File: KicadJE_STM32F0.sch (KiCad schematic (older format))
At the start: 101 parts, among them J401 CV1, J402 CV2, J403 OUT1, J404 OUT2, J405 OUT3, J406 OUT4, J407 IN1, J408 IN2, J409 I2C, P401 Doepfer_Power_16pin, SW401 SW_SPDT, U401 TL072, U402 TL072, U405 MCP4822

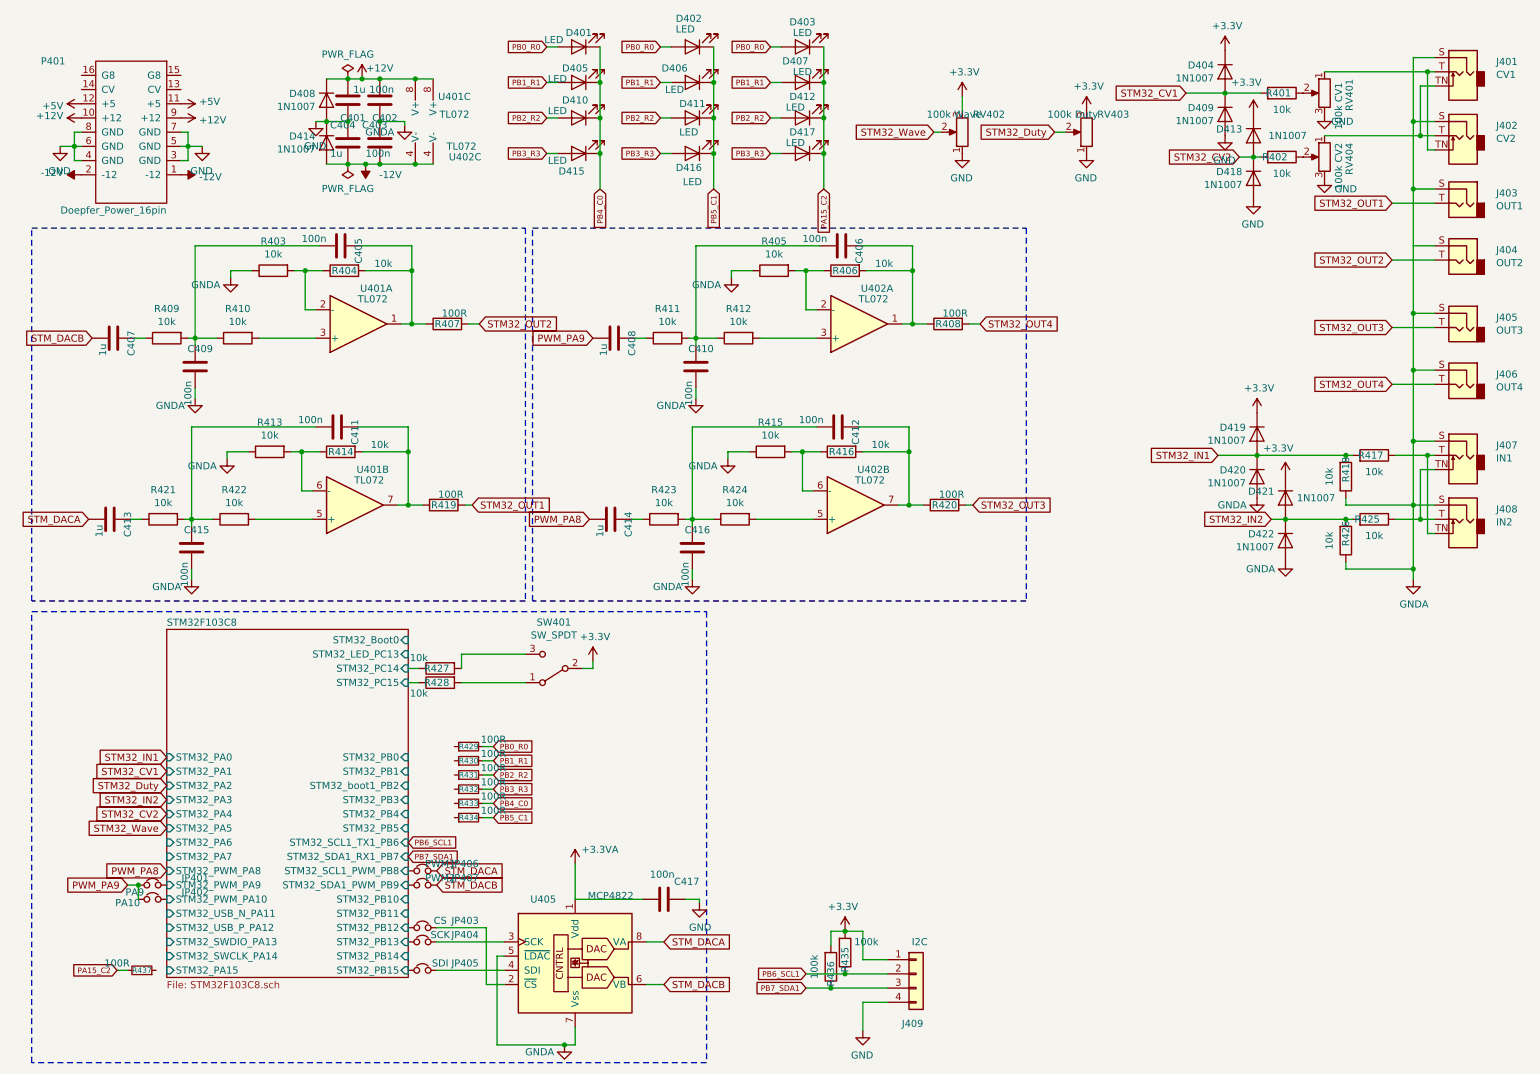
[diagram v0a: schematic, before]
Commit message: Diode etc
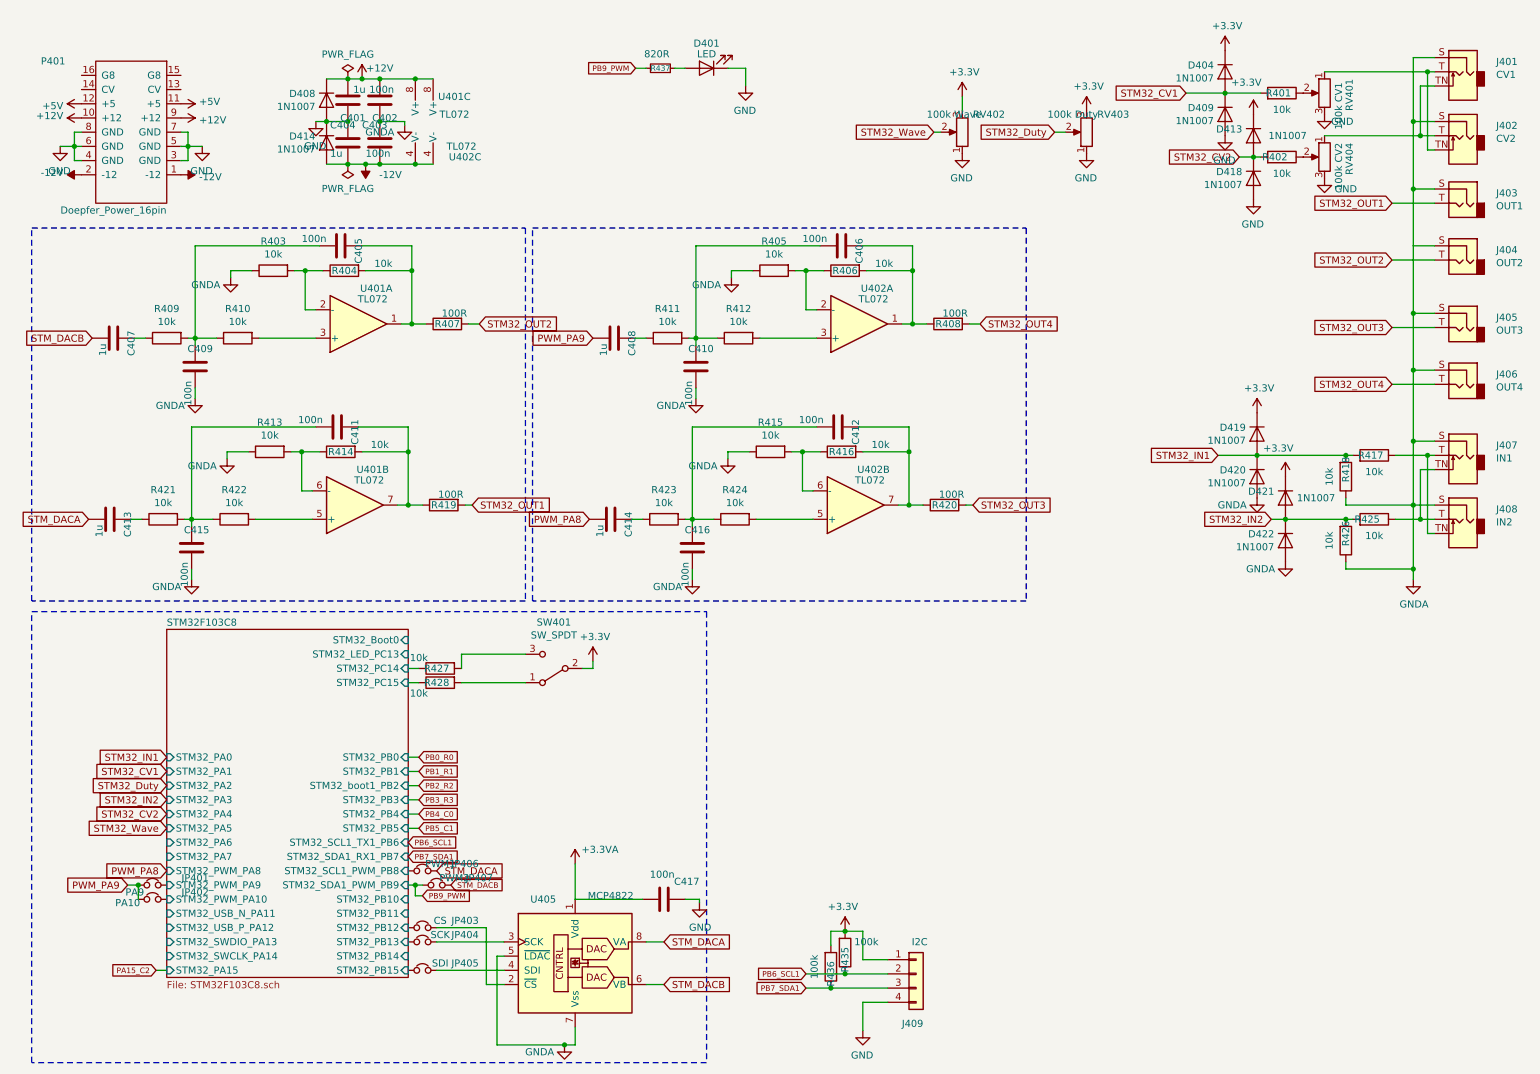
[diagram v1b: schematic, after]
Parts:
- removed D401, D402, D405, D406, D407, D410, D411, D412, D415, D416, D417: LED, LED_THT:LED_D3.0mm, symbol Device:LED
- removed R429, R430, R431, R432, R433, R434: 100R, Resistor_SMD:R_0805_2012Metric_Pad1.15x1.40mm_HandSolder, symbol Device:R_Small
- R437: value 100R -> 820R
- renumbered D403 to D401
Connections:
- net GND: now also D401.1 (K)
- net PA15_C2: no longer D401.1 (K), R437.2
- net PB0_R0: no longer D401.2 (A)
- net at R437.1: now also D401.2 (A)
- net STM32F103C8/STM32_SDA1_PWM_PB9 renamed PB9_PWM
- net PB9_PWM: now also R437.2
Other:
- moved on the sheet: D401, JP407, R437
